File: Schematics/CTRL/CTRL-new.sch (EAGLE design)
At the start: 117 parts

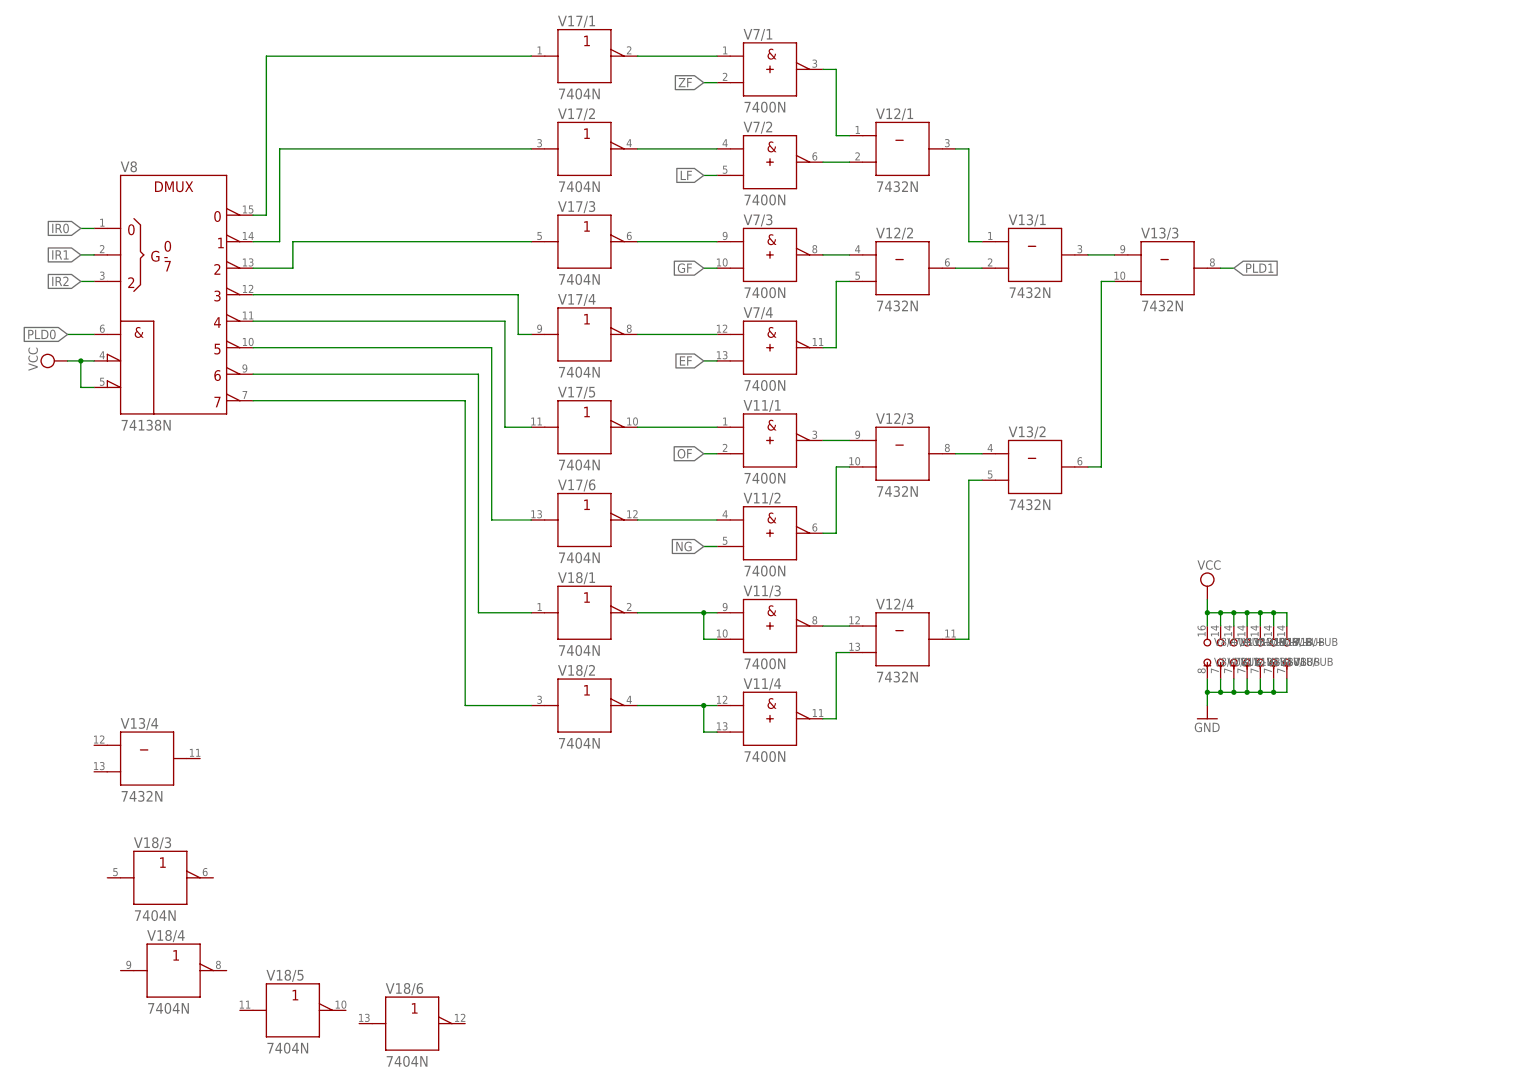
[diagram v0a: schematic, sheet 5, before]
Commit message: fixed PLD
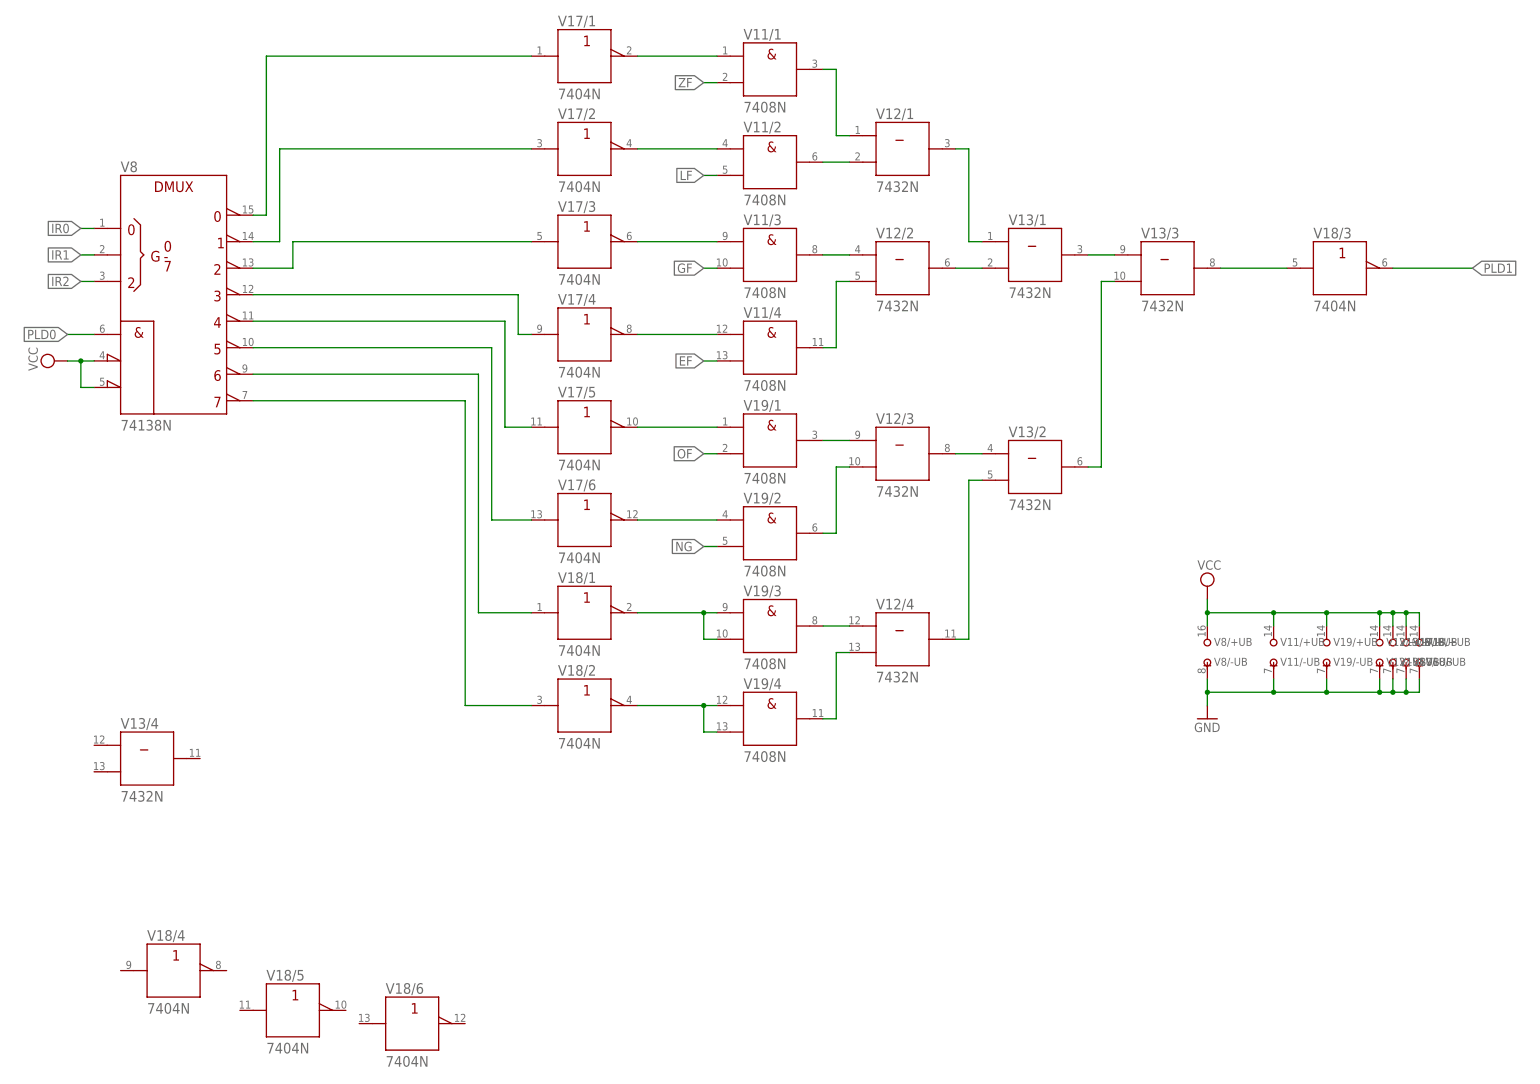
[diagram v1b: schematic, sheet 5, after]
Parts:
- removed V7: 7400N, 74ttl-din:7400N
- added V19: 7408N, 74ttl-din:7408N
- V11: value 7400N -> 7408N; device 74ttl-din:7400N -> 74ttl-din:7408N
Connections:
- new net N$54: V13/3.Y, V18/3.A
- net EF: now also V11/4.B; no longer V7/4.B
- net GF: now also V11/3.B; no longer V7/3.B
- net GND: now also V19/-UB.-UB; no longer V7/-UB.-UB
- net LF: now also V11/2.B; no longer V7/2.B
- net N$100: now also V19/3.Y; no longer V11/3.Y
- net N$14: now also V19/3.A, V19/3.B; no longer V11/3.A, V11/3.B
- net N$34: now also V19/4.A, V19/4.B; no longer V11/4.A, V11/4.B
- net N$35: now also V19/2.A; no longer V11/2.A
- net N$36: now also V19/1.A; no longer V11/1.A
- net N$37: now also V11/4.A; no longer V7/4.A
- net N$38: now also V11/3.A; no longer V7/3.A
- net N$39: now also V11/2.A; no longer V7/2.A
- net N$40: now also V11/1.A; no longer V7/1.A
- net N$89: now also V11/1.Y; no longer V7/1.Y
- net N$90: now also V11/2.Y; no longer V7/2.Y
- net N$91: now also V11/3.Y; no longer V7/3.Y
- net N$92: now also V11/4.Y; no longer V7/4.Y
- net N$93: now also V19/1.Y; no longer V11/1.Y
- net N$94: now also V19/2.Y; no longer V11/2.Y
- net N$99: now also V19/4.Y; no longer V11/4.Y
- net NG: now also V19/2.B; no longer V11/2.B
- net OF: now also V19/1.B; no longer V11/1.B
- net PLD1: now also V18/3.Y; no longer V13/3.Y
- net VCC: now also V19/+UB.+UB; no longer V7/+UB.+UB
- net ZF: now also V11/1.B; no longer V7/1.B
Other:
- moved on the sheet: V11/+UB, V11/-UB, V12/+UB, V12/-UB, V13/+UB, V13/-UB, V17/+UB, V17/-UB, V18/+UB, V18/-UB, V18/3
